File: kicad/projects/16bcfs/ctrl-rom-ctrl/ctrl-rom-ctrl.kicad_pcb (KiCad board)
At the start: 4 copper layers, 88.9 x 43.2 mm, 104 parts, among them J1 Instruction, J2 Control ROM Address, J3 Raw Address for Pgm ROM, J4 Signal Header, J5 Power, J6 Power, U1 74HC08, U11 74HC157, U12 74HC157, U13 74HC157, U14 74HC157, U15 74HC193, U16 74HC193, U17 74HC193, U18 74HC193, U19 74HC04, U2 74HC74, U21 74HC08, U22 74HC08, U23 74HC32, U3 74HC03, U4 74HC193, U5 74HC541, U6 74HC00, U7 74HC00, U8 74HC541, U9 74HC165, X1 XO32

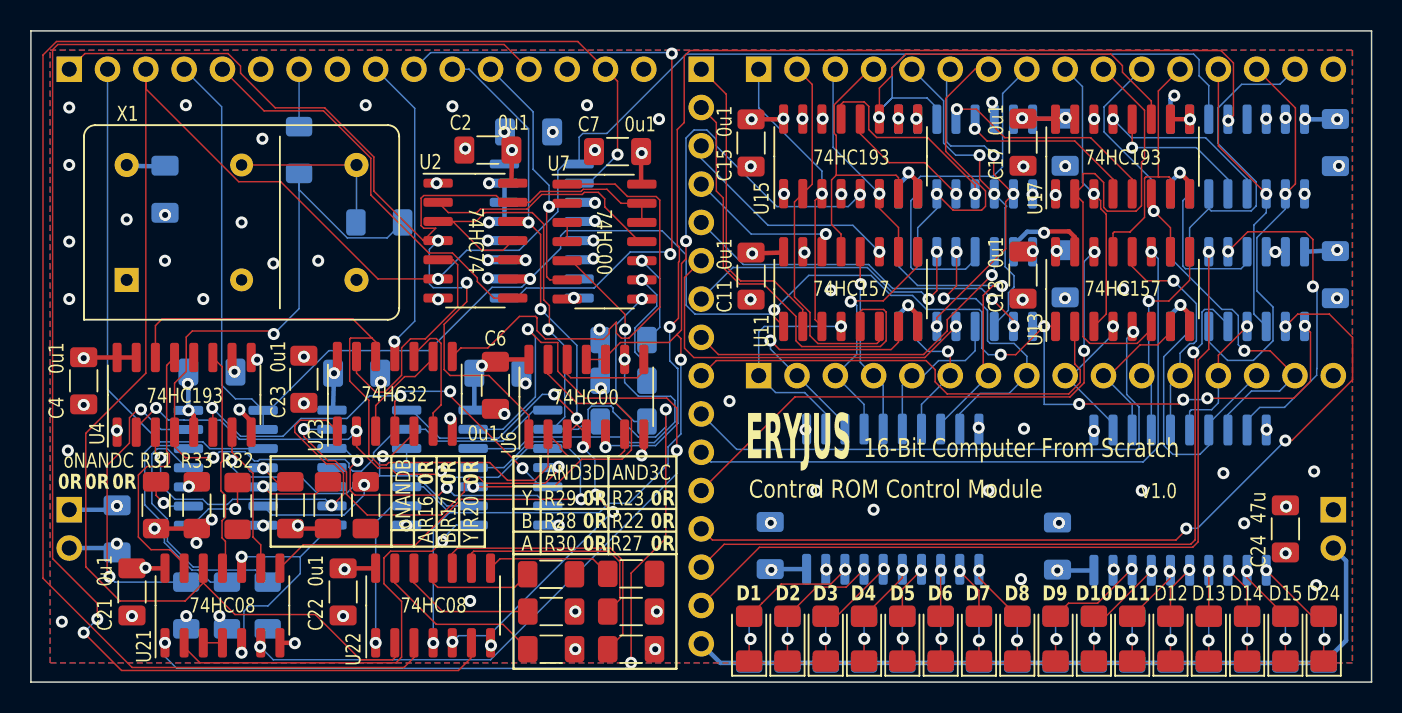
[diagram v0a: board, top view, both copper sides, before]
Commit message: Clean up some remaining comments
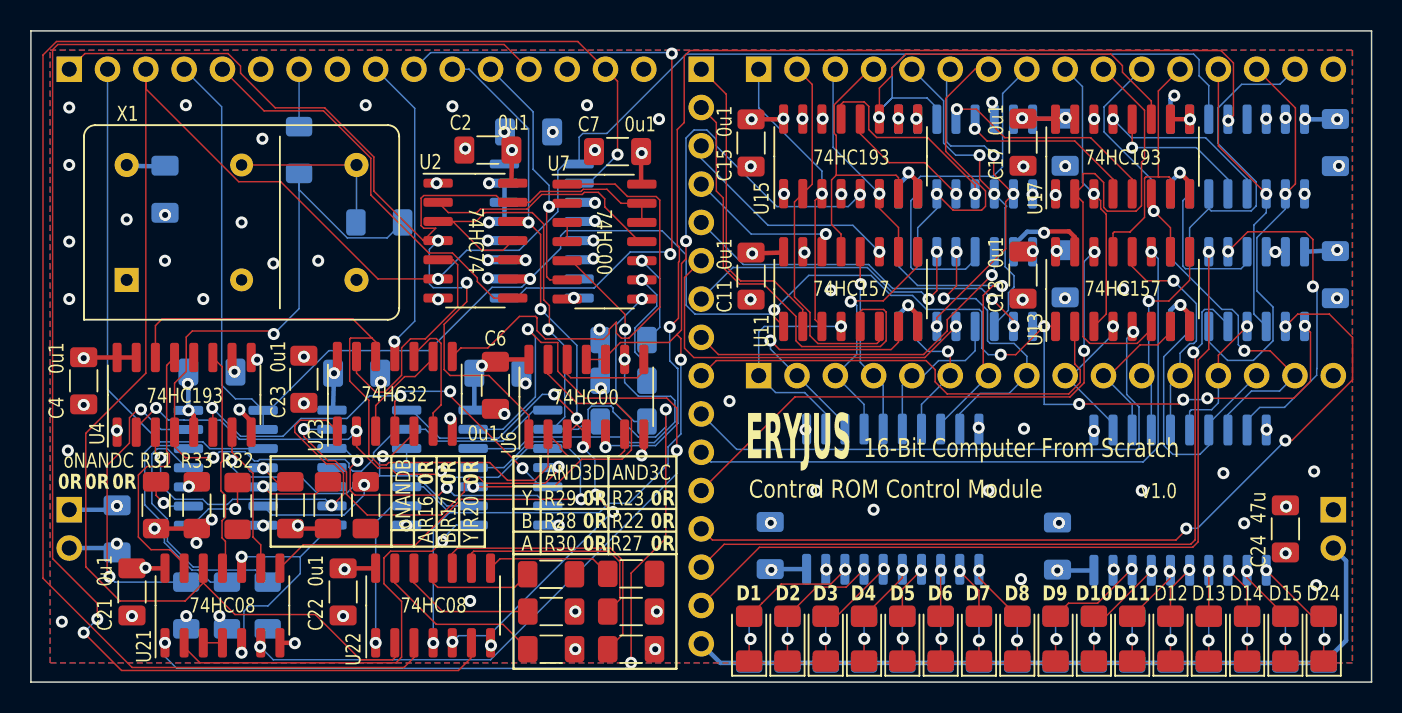
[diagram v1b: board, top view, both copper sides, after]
